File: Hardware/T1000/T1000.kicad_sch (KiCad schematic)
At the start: 76 parts, among them J1 USB_C_Receptacle_USB2.0, J2 SOICbite, Q1 IRLML0060TRPBF, U2 RP2040, U3 W25Q128JVS, U4 LTC4419, U5 MAX-M10S, U6 MS5607-02BA, U7 LT6703CDC-3, U8 MAX77857, Y1 445I23D12M00000

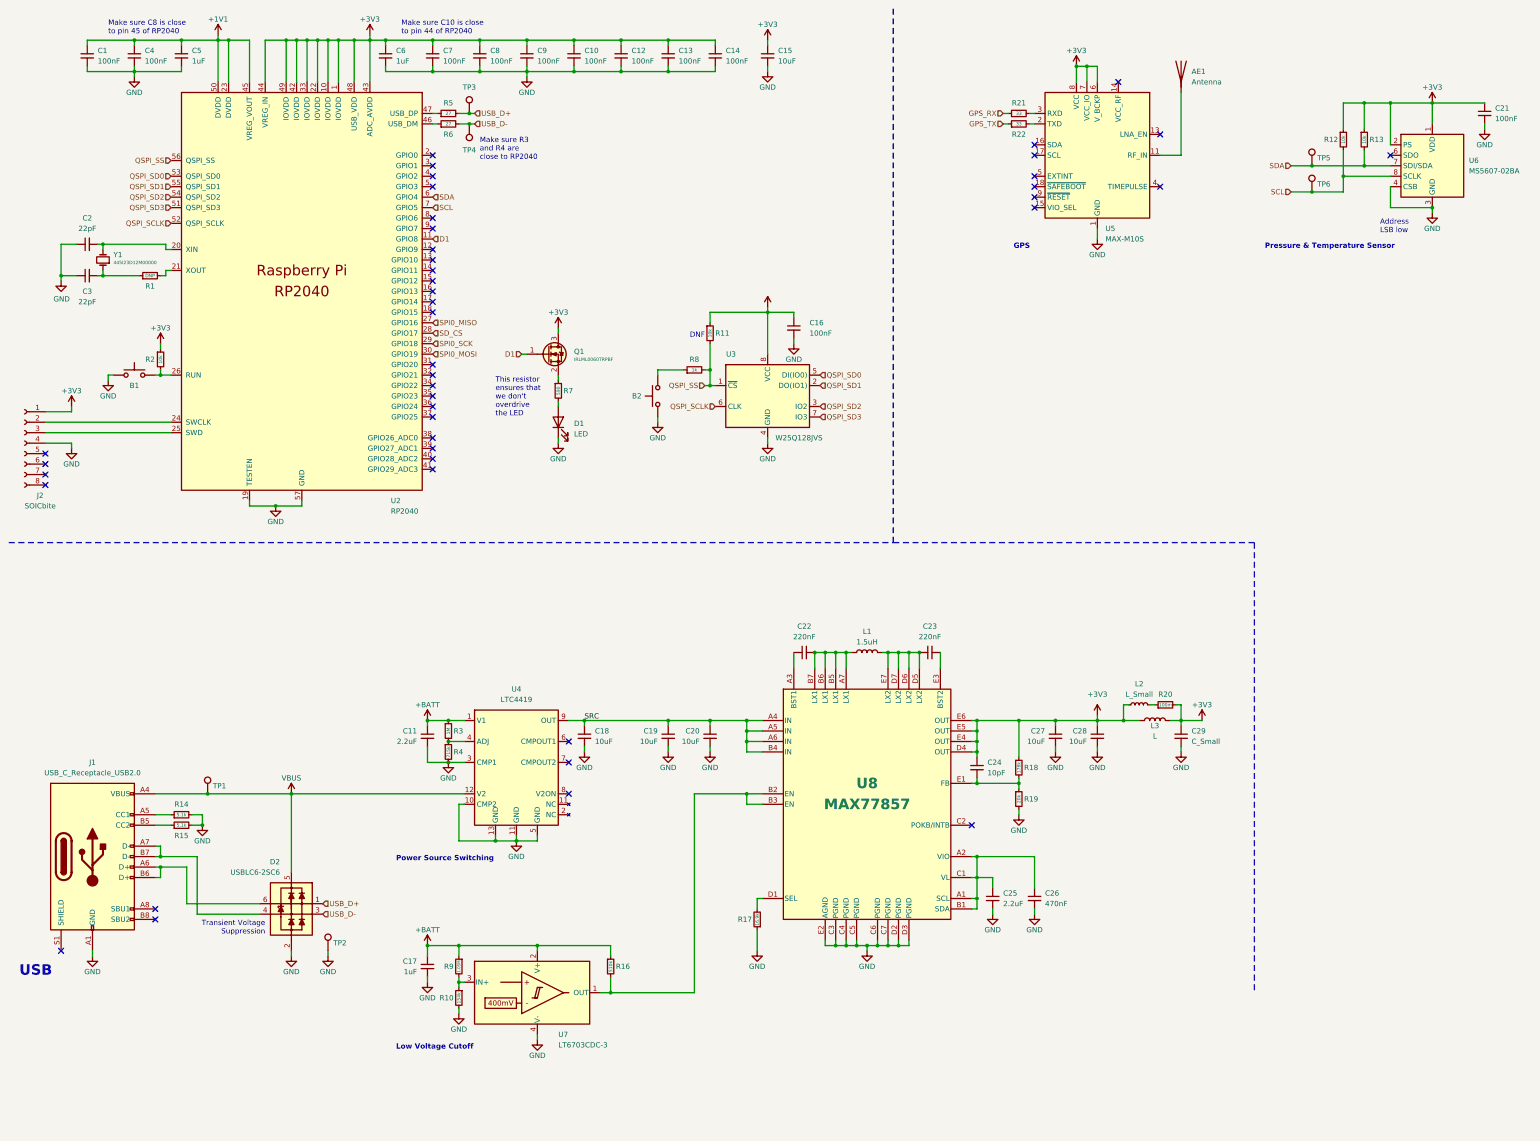
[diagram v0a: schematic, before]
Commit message: filter tuning
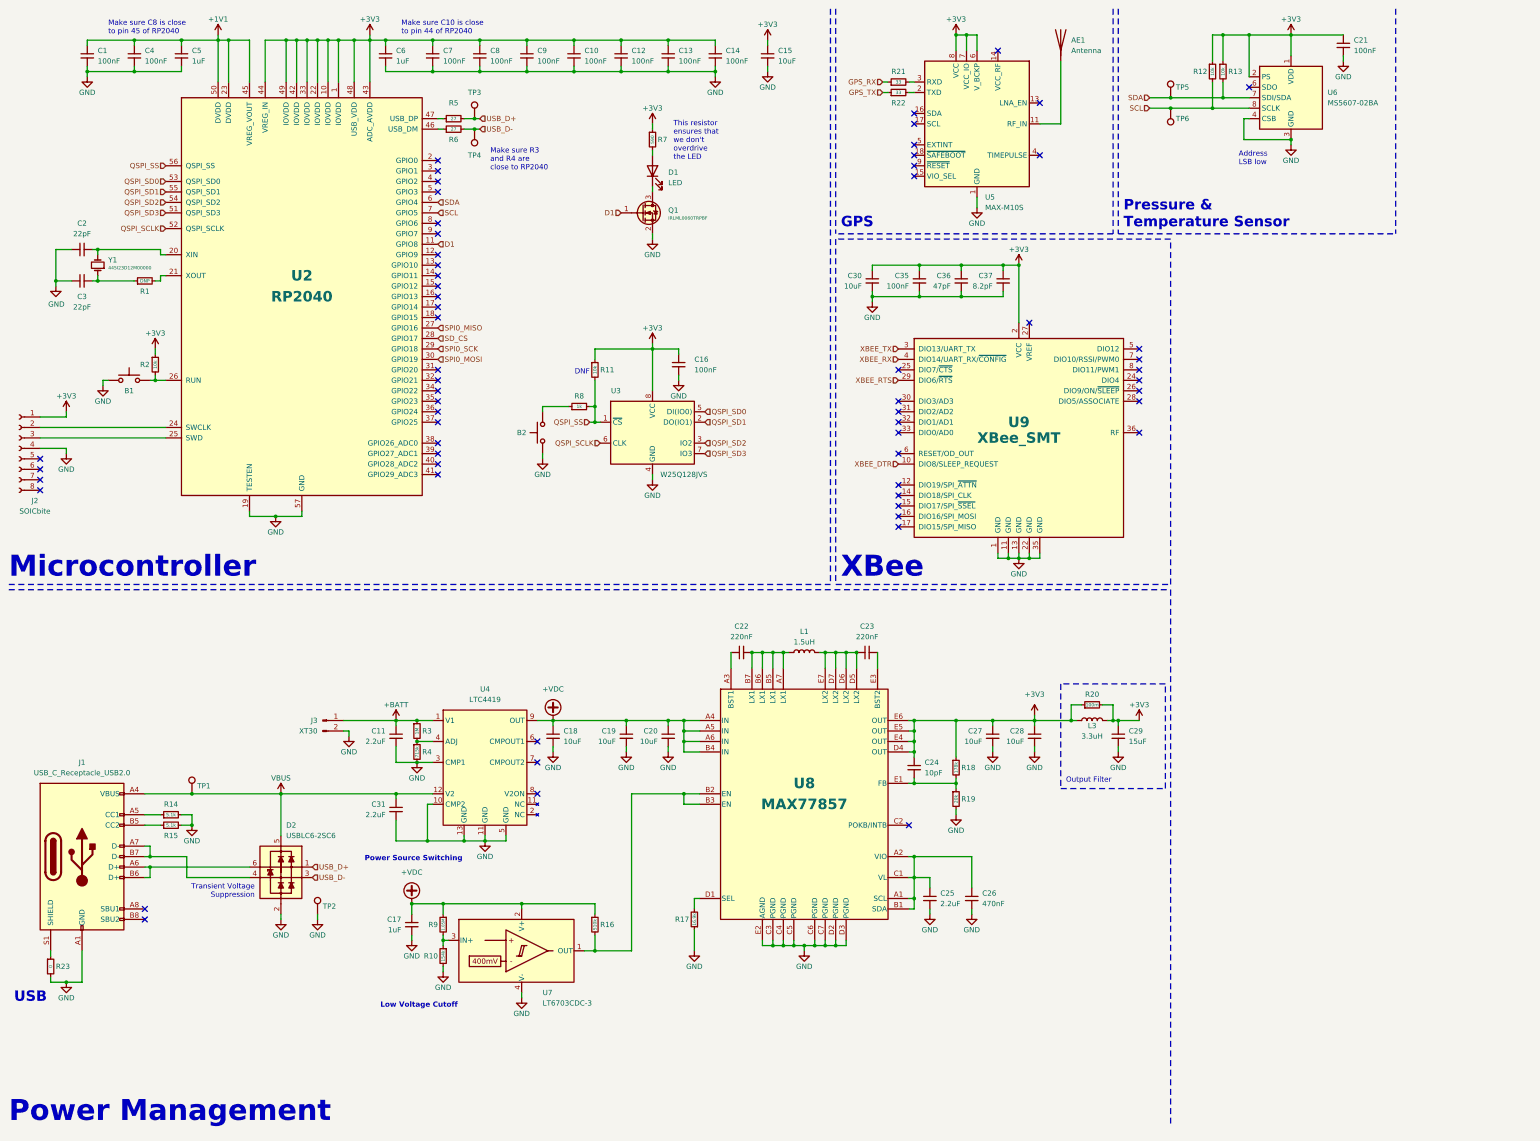
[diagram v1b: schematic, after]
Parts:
- removed L2: L_Small, symbol Device:L_Small
- added C30: 10uF, symbol Device:C_Small
- added C31: 2.2uF, Capacitor_SMD:C_0603_1608Metric_Pad1.08x0.95mm_HandSolder, symbol Device:C_Small
- added C35: 100nF, symbol Device:C_Small
- added C36: 47pF, symbol Device:C_Small
- added C37: 8.2pF, symbol Device:C_Small
- added J3: XT30, symbol Connector:Conn_01x02_Pin
- added R23: 0, symbol Device:R_Small
- added U9: XBee_SMT, RF_Module:Digi_XBee_SMT, symbol RF_ZigBee:XBee_SMT
- C29: value C_Small -> 15uF
- L3: value L -> 3.3uH
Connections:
- net +3V3: now also R20.1, R7.1, C30.1, C35.1, C36.1, C37.1, U9.2 (VCC); no longer Q1.3 (D)
- net +BATT: now also J3.1 (Pin_1); no longer C17.1, R16.1, R9.1, U7.2 (V+)
- net GND: now also Q1.2 (S), C30.2, C31.2, C35.2, C36.2, C37.2, J3.2 (Pin_2), R23.2, U9.1 (GND), U9.11 (GND), U9.13 (GND), U9.22 (GND), U9.35 (GND); no longer D1.1 (K)
- net VBUS: now also C31.1
- net at J1.S1 (SHIELD): now also R23.1
- net SRC renamed +VDC
- net +VDC: now also C17.1, R16.1, R9.1, U7.2 (V+)
- new net: D1.1 (K), Q1.3 (D)
- new net XBEE_DTR: U9.10 (DIO8/SLEEP_REQUEST)
- new net XBEE_RTS: U9.29 (DIO6/~{RTS})
- new net XBEE_RX: U9.4 (DIO14/UART_RX/~{CONFIG})
- new net XBEE_TX: U9.3 (DIO13/UART_TX)
- no-connect marks 44 -> 62
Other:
- note added: "Microcontroller"
- note added: "Output Filter"
- note added: "Power Management"
- note added: "XBee"
- moved on the sheet: AE1, B1, B2, C11, C16, C17, C18, C19, C2, C20, C21, C22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
